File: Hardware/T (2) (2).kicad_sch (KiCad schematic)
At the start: 25 parts, among them J1 SHARP 1, J2 BTS-1, J3 SHARP2, J4 SHARP 3, J5 BTS-2, J6 QTR8A, J7 SHARP 5, J8 SHARP4, SW1 SW_DPST_x2, SW2 BOTON, U2 AMS1117-3.3

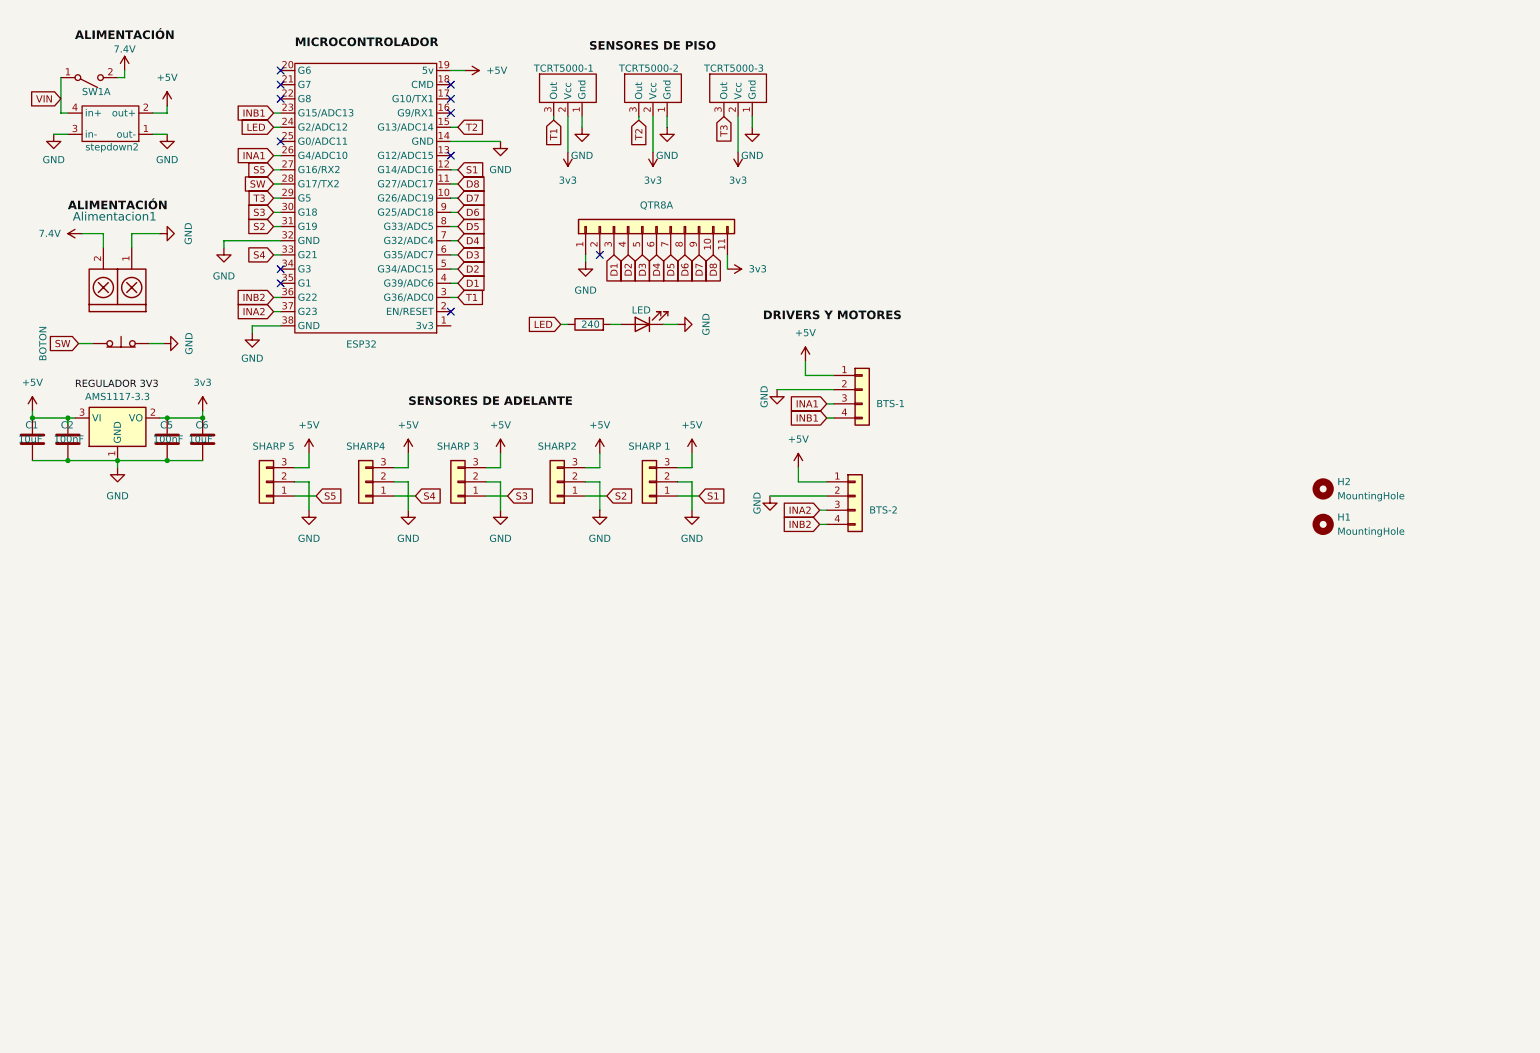
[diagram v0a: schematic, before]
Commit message: Add files via upload
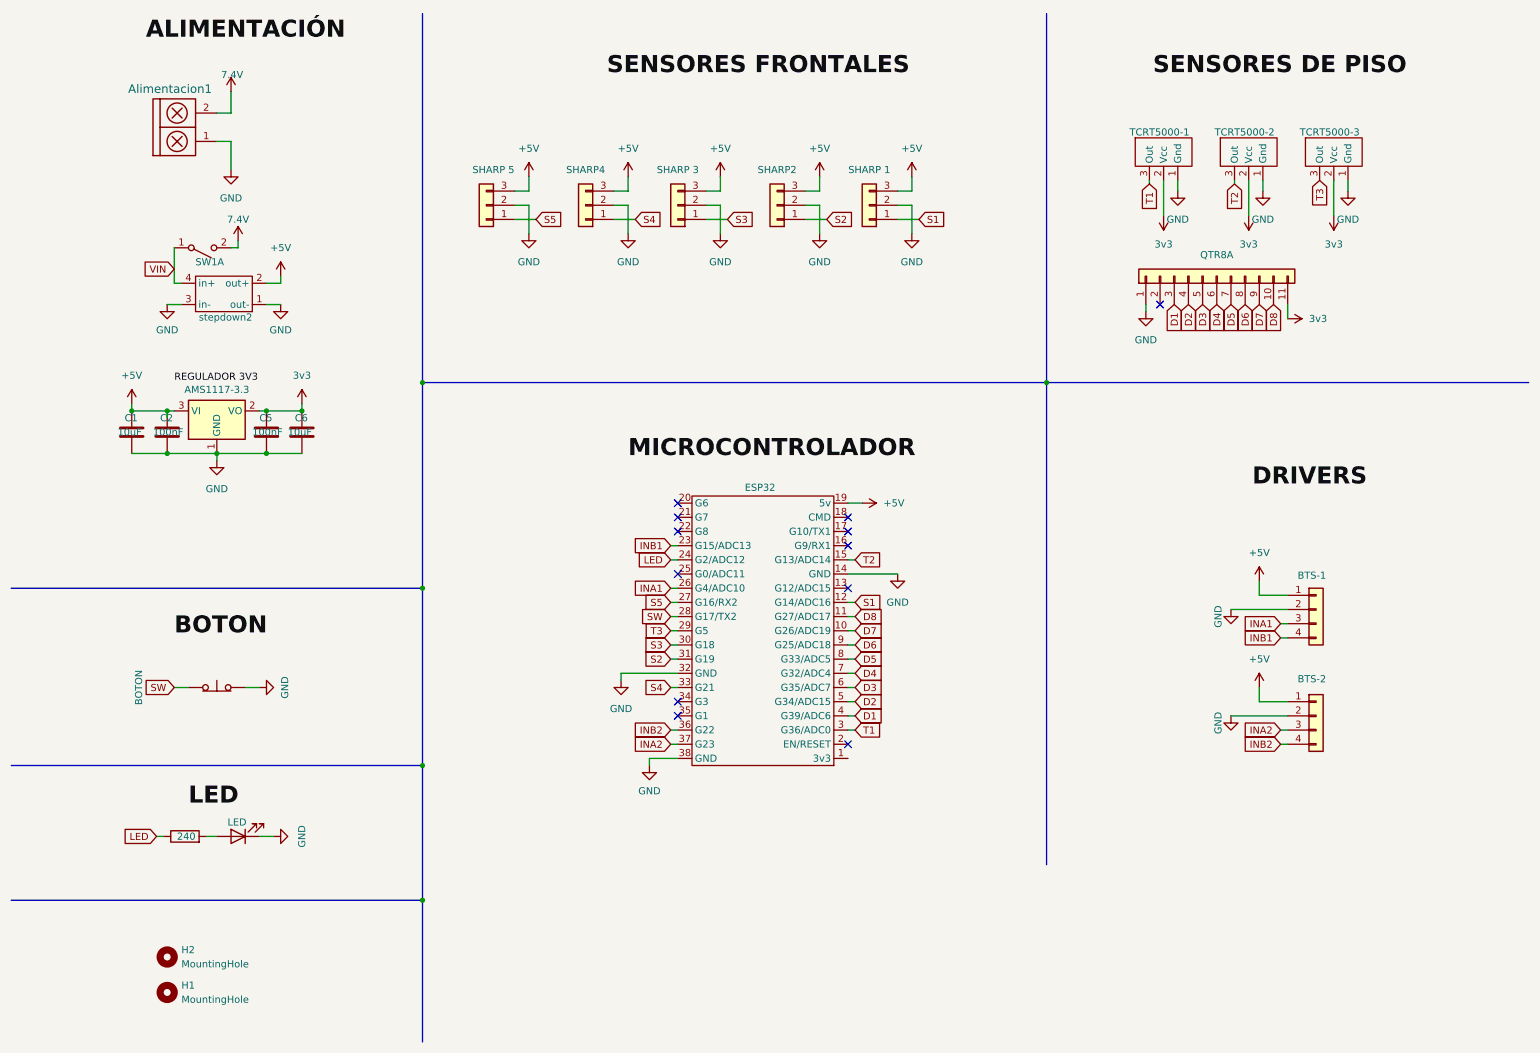
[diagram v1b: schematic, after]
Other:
- moved on the sheet: Alimentacion1, C1, C2, C5, C6, ESP32, H1, H2, SW1A, TCRT5000-1, TCRT5000-2, TCRT5000-3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
